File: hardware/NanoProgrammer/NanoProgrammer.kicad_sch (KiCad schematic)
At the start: 20 parts, among them J1 USB_A, J3 Conn_01x05, J4 Conn_01x04, U1 DS2480B+, U2 HT42B534

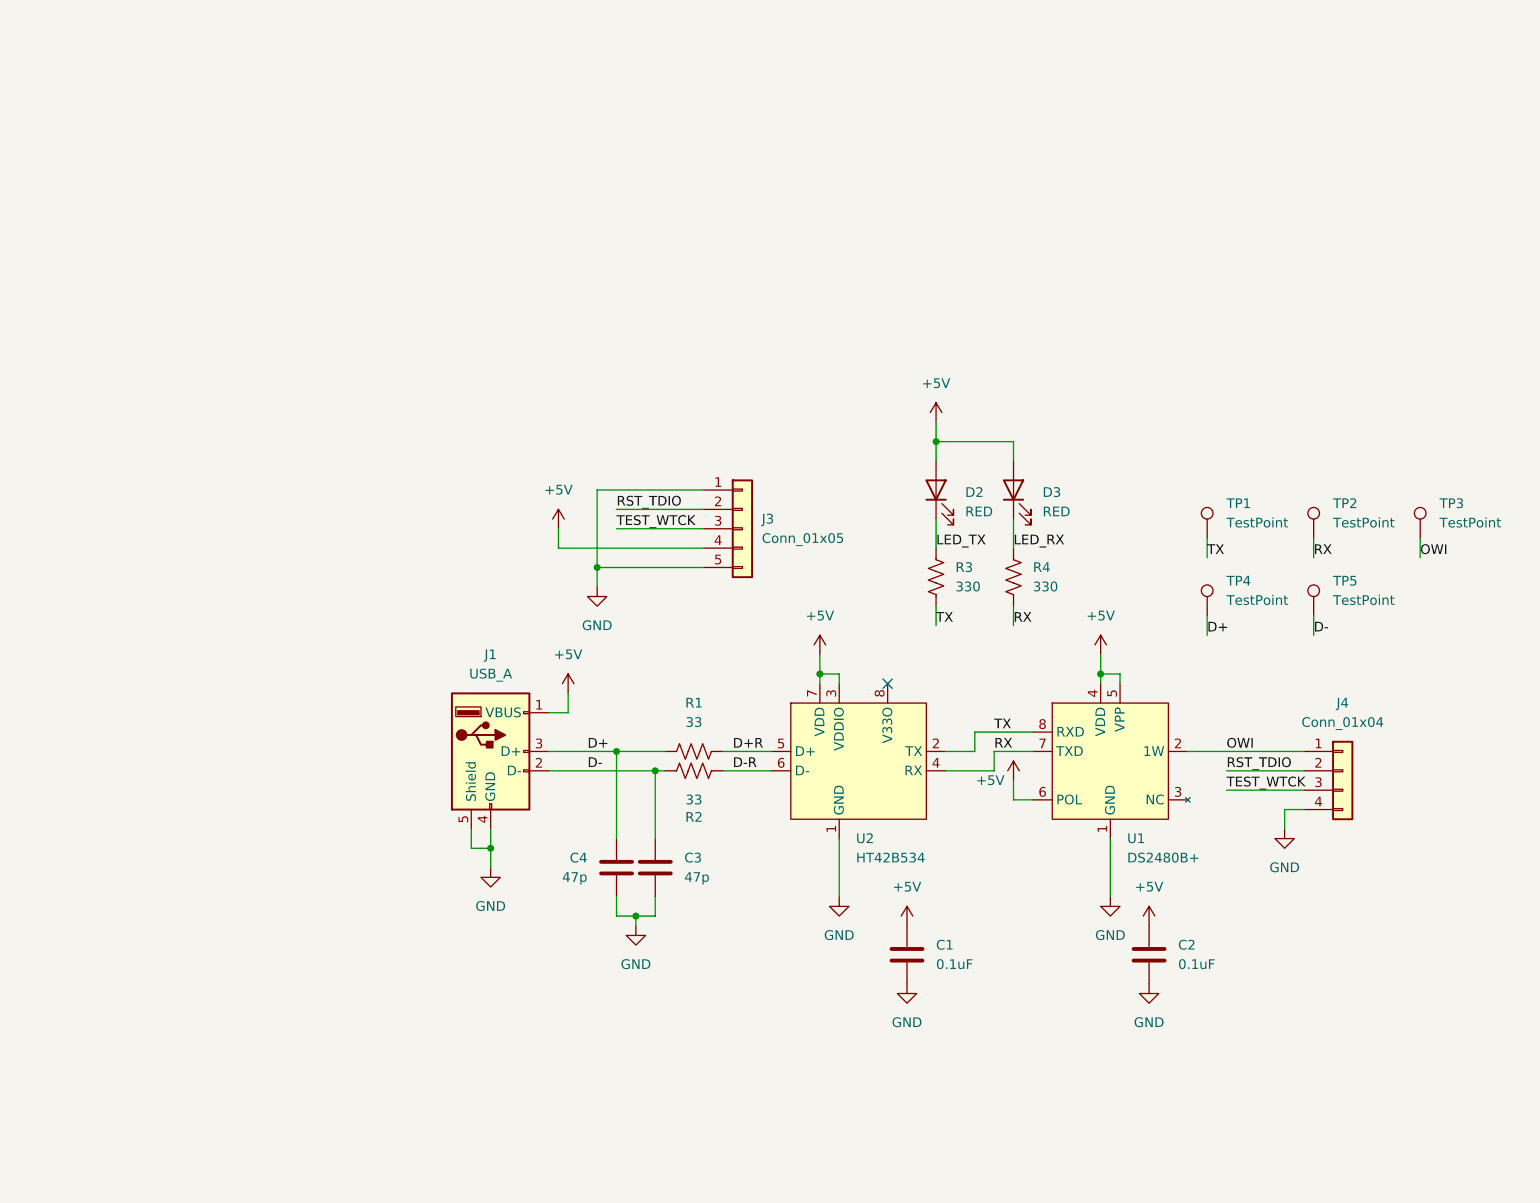
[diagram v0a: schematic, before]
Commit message: huge bunch of uncommitted stuff idk what this is
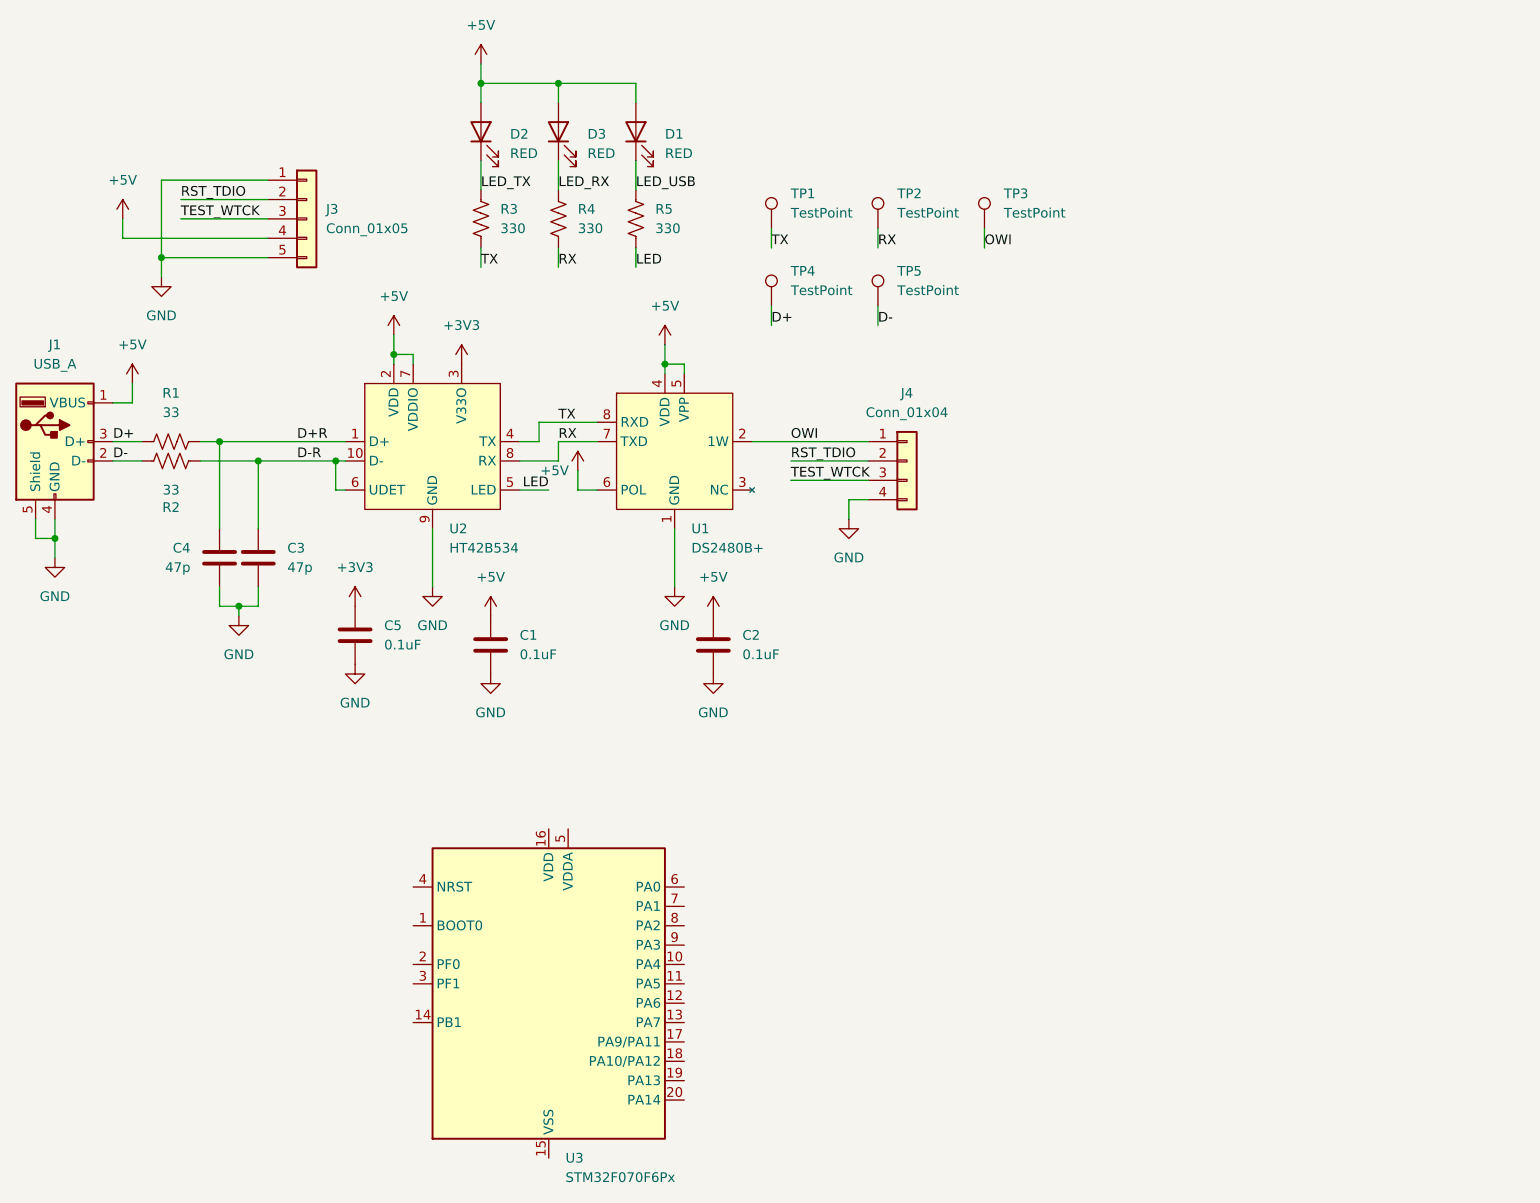
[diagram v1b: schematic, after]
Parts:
- removed U2: HT42B534, Package_SO:SO-8_3.9x4.9mm_P1.27mm, symbol Interface_Custom:HT42B534-02_8SOP
- added C5: 0.1uF, Capacitor_SMD:C_0402_1005Metric, symbol Device:C
- added D1: RED, LED_SMD:LED_0603_1608Metric, symbol Device:LED
- added R5: 330, Resistor_SMD:R_0402_1005Metric, symbol Device:R_US
- added U2: HT42B534, Package_SO:SSOP-10_3.9x4.9mm_P1.00mm, symbol Interface_Custom:HT42B534-02_10SOP
- added U3: STM32F070F6Px, Package_SO:TSSOP-20_4.4x6.5mm_P0.65mm, symbol MCU_ST_STM32F0:STM32F070F6Px
- U1: JLCPCB_CORRECTION 0;0;90 -> 0;0;-90
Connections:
- net +5V: now also D1.2 (A), U2.2 (VDD), U2.7 (VDDIO)
- net D+: no longer C4.1
- net D+R: now also C4.1, U2.1 (D+)
- net D-: no longer C3.1
- net D-R: now also C3.1, U2.10 (D-), U2.6 (UDET)
- net GND: now also C5.2, U2.9 (GND)
- net RX: now also U2.8 (RX)
- net TX: now also U2.4 (TX)
- new net +3V3: C5.1, U2.3 (V33O)
- new net LED: R5.1, U2.5 (LED)
- new net LED_USB: D1.1 (K), R5.2
- no-connect marks 1 -> 0
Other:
- moved on the sheet: C1, C2, C3, C4, D2, D3, J1, J3, J4, R1, R2, R3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
